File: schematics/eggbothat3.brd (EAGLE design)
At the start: 100.2 x 80 mm, 43 parts

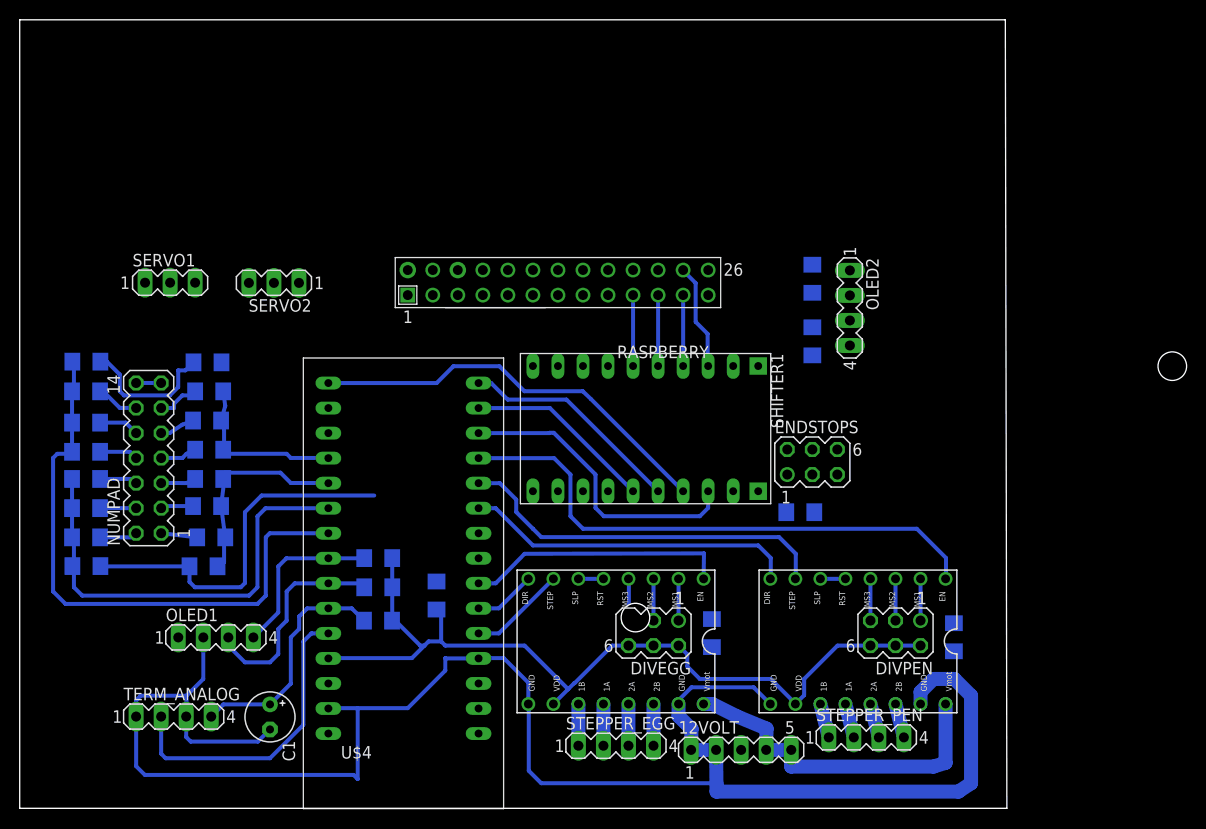
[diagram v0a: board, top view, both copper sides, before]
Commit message: versions 2,3 of electronics
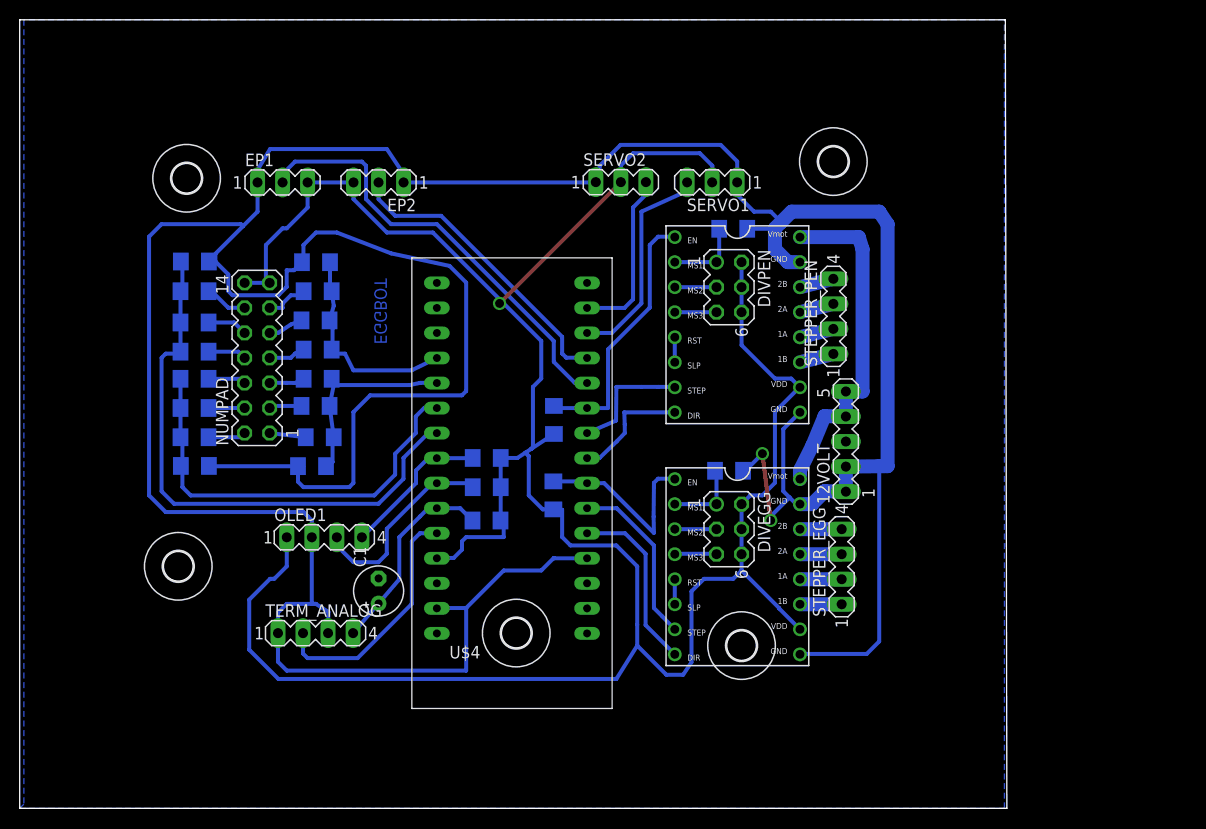
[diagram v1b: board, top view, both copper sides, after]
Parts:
- removed ENDSTOPS: (no value), con-lstb:MA03-2
- removed OLED2: (no value), con-lstb:MA04-1
- removed R8, R9: 4k7, rcl:R1206
- removed RASPBERRY: RPI-B-V2SHIELD, levelshifter:RPI-B-V2-SHIELD
- removed SHIFTER1: LEVELSHIFTER, levelshifter:PLUG_20_S4
- added EP1, EP2: (no value), con-lstb:MA03-1
- added U$3, U$5, U$6, U$7, U$8: (no value), holes:3,0
- moved SERVO1 55.9 mm to (70.3, 63.5), turned to 180 degrees
- moved U$1 47.2 mm to (77.9, 56.7), turned to 270 degrees
- moved R2 47.1 mm to (72.4, 58.8), turned to 180 degrees
- moved STEPPER_PEN 42.8 mm to (82.6, 49.9), turned to 90 degrees
- moved DIVPEN 38.9 mm to (72.0, 52.9), turned to 270 degrees
- moved SERVO2 36.7 mm to (61.0, 63.5), turned to 0 degrees
- moved 12VOLT 33.0 mm to (83.8, 37.2), turned to 90 degrees
- moved STEPPER_EGG 29.2 mm to (83.4, 24.5), turned to 90 degrees
- moved R11 26.7 mm to (54.2, 39.4), turned to 270 degrees
- moved U$2 22.5 mm to (77.9, 32.1), turned to 270 degrees
- moved C1 16.9 mm to (36.4, 22.1), turned to 90 degrees
- moved TERM_ANALOG 16.7 mm to (30.0, 17.8)
- moved R3 16.6 mm to (72.0, 34.2), turned to 180 degrees
- moved R12 15.6 mm to (54.1, 31.7)
- moved R10 15.0 mm to (47.4, 29.2)
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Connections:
- removed net +3V3: ENDSTOPS.5, ENDSTOPS.6, OLED2.1, R8.2, R9.2, RASPBERRY.P1_1, RASPBERRY.P1_17, SHIFTER1.VCCA
- removed net I2C2_SCL: OLED2.3, R9.1, RASPBERRY.P1_5
- removed net I2C2_SDA: OLED2.4, R8.1, RASPBERRY.P1_3
- removed net SPI33_CLK: RASPBERRY.P1_23, SHIFTER1.A3
- removed net SPI33_CS1: RASPBERRY.P1_24, SHIFTER1.A2
- removed net SPI33_MISO: RASPBERRY.P1_21, SHIFTER1.A4
- removed net SPI33_MOSI: RASPBERRY.P1_19, SHIFTER1.A5
- removed net SPI_CLK: SHIFTER1.B3, U$4.D13
- removed net SPI_CS1: SHIFTER1.B2, U$4.D10
- removed net SPI_MISO: SHIFTER1.B4, U$4.D12
- removed net SPI_MOSI: SHIFTER1.B5, U$4.D11
- new net LED-INTERN: U$4.D13
- new net NC1: U$4.D12
- net E-DIR: now also U$4.D2; no longer U$4.D3
- net E-STEP: now also U$4.D3; no longer U$4.D2
- net END1: now also EP1.2, U$4.D8; no longer ENDSTOPS.4, RASPBERRY.P1_8
- net END2: now also EP2.2, U$4.D9; no longer ENDSTOPS.3, RASPBERRY.P1_10
- net GND: now also EP1.1, EP2.1; no longer ENDSTOPS.1, ENDSTOPS.2, OLED2.2, RASPBERRY.P1_14, RASPBERRY.P1_20, RASPBERRY.P1_25, RASPBERRY.P1_6, RASPBERRY.P1_9, SHIFTER1.GND
- net P-DIR: now also U$4.D5; no longer U$4.D7
- net P-EN: now also U$4.D7; no longer U$4.D9
- net P-STEP: now also U$4.D6; no longer U$4.D8
- net PWM1: now also U$4.D10; no longer U$4.D5
- net PWM2: now also U$4.D11; no longer U$4.D6
- net VCC: now also EP1.3, EP2.3; no longer RASPBERRY.P1_2, RASPBERRY.P1_4, SHIFTER1.VCCB
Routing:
- net VCC: track 90.0 -> 263.2 mm, vias 0 -> 1
- net GND: track 233.5 -> 384.0 mm, vias 0 -> 2
- net END1: track 0.00 -> 44.8 mm
- net SPI_CLK: track 41.9 -> 0.00 mm
- net SPI_CS1: track 30.8 -> 0.00 mm
- net END2: track 0.00 -> 30.5 mm
- net P-EN: track 56.2 -> 26.7 mm
- net P-STEP: track 38.5 -> 12.6 mm
- net SPI_MISO: track 22.8 -> 0.00 mm
- net PWM1: track 0.00 -> 22.0 mm
- net P-DIR: track 33.9 -> 12.1 mm
- net SPI_MOSI: track 19.2 -> 0.00 mm
- net PWM2: track 0.00 -> 17.5 mm
- net E-DIR: track 6.29 -> 18.2 mm
- net SPI33_CS1: track 10.8 -> 0.00 mm
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- added copper zone on layer 16, net GND
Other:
- board text added: "EGGBOT"
